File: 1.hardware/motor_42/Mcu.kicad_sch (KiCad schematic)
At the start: 0 parts

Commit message: 중간 저장
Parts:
- added U1: STM32F103CBTx, Package_QFP:LQFP-48_7x7mm_P0.5mm, symbol MCU_ST_STM32F1:STM32F103CBTx
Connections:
- new net: U1.23 (VSS), U1.35 (VSS), U1.47 (VSS)
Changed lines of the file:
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@@
 (kicad_sch
-	(version 20231120)
+	(version 20250114)
 	(generator "eeschema")
-	(generator_version "8.0")
+	(generator_version "9.0")
 	(paper "A4")
+	(symbol
+		(lib_id "MCU_ST_STM32F1:STM32F103CBTx")
+		(at 154.94 92.71 0)
+		(unit 1)
+		(exclude_from_sim no)
+		(in_bom yes)
+		(on_board yes)
+		(dnp no)
+		(fields_autoplaced yes)
+		(property "Reference" "U1"
+			(at 159.6233 133.35 0)
+			(effects
+				(font
+					(size 1.27 1.27)
+				)
+				(justify left)
+			)
+		)
+		(property "Value" "STM32F103CBTx"
+			(at 159.6233 135.89 0)
+			(effects
+				(font
+					(size 1.27 1.27)
+				)
+				(justify left)
+			)
+		)
+		(property "Footprint" "Package_QFP:LQFP-48_7x7mm_P0.5mm"
+			(at 139.7 130.81 0)
+			(effects
+				(font
+					(size 1.27 1.27)
+				)
+				(justify right)
+				(hide yes)
+			)
+		)
+		(property "Datasheet" "https://www.st.com/resource/en/datasheet/stm32f103cb.pdf"
+			(at 154.94 92.71 0)
+			(effects
+				(font
+					(size 1.27 1.27)
+				)
+				(hide yes)
+			)
+		)
+		(property "Description" "STMicroelectronics Arm Cortex-M3 MCU, 128KB flash, 20KB RAM, 72 MHz, 2.0-3.6V, 37 GPIO, LQFP48"
+			(at 154.94 92.71 0)
+			(effects
+				(font
+					(size 1.27 1.27)
+				)
+				(hide yes)
+			)
+		)
+		(pin "18"
+		)
+		(pin "43"
+		)
+		(pin "39"
+		)
+		(pin "24"
+		)
+		(pin "36"
+		)
+		(pin "47"
+		)
+		(pin "1"
+		)
+		(pin "46"
+		)
+		(pin "45"
+		)
+		(pin "27"
+		)
+		(pin "8"
+		)
+		(pin "28"
+		)
+		(pin "21"
+		)
+		(pin "26"
+		)
+		(pin "6"
+		)
+		(pin "3"
+		)
+		(pin "4"
+		)
+		(pin "2"
+		)
+		(pin "19"
+		)
+		(pin "40"
+		)
+		(pin "41"
+		)
+		(pin "5"
+		)
+		(pin "42"
+		)
+		(pin "44"
+		)
+		(pin "7"
+		)
+		(pin "20"
+		)
+		(pin "22"
+		)
+		(pin "25"
+		)
+		(pin "23"
+		)
+		(pin "35"
+		)
+		(pin "48"
+		)
+		(pin "13"
+		)
+		(pin "32"
+		)
+		(pin "31"
+		)
+		(pin "29"
+		)
+		(pin "14"
+		)
+		(pin "17"
+		)
+		(pin "34"
+		)
+		(pin "16"
+		)
+		(pin "38"
+		)
+		(pin "15"
+		)
+		(pin "11"
+		)
+		(pin "30"
+		)
+		(pin "10"
+		)
+		(pin "12"
+		)
+		(pin "33"
+		)
+		(pin "37"
+		)
+		(pin "9"
+		)
+		(instances
+			(project ""
+				(path "/3c5de6a8-6840-43a5-a2fb-24dbb7f0450d/91ecfca5-1fde-4bfb-b396-1bb710e5b1bd"
+					(reference "U1")
+					(unit 1)
+				)
+			)
+		)
+	)
 )

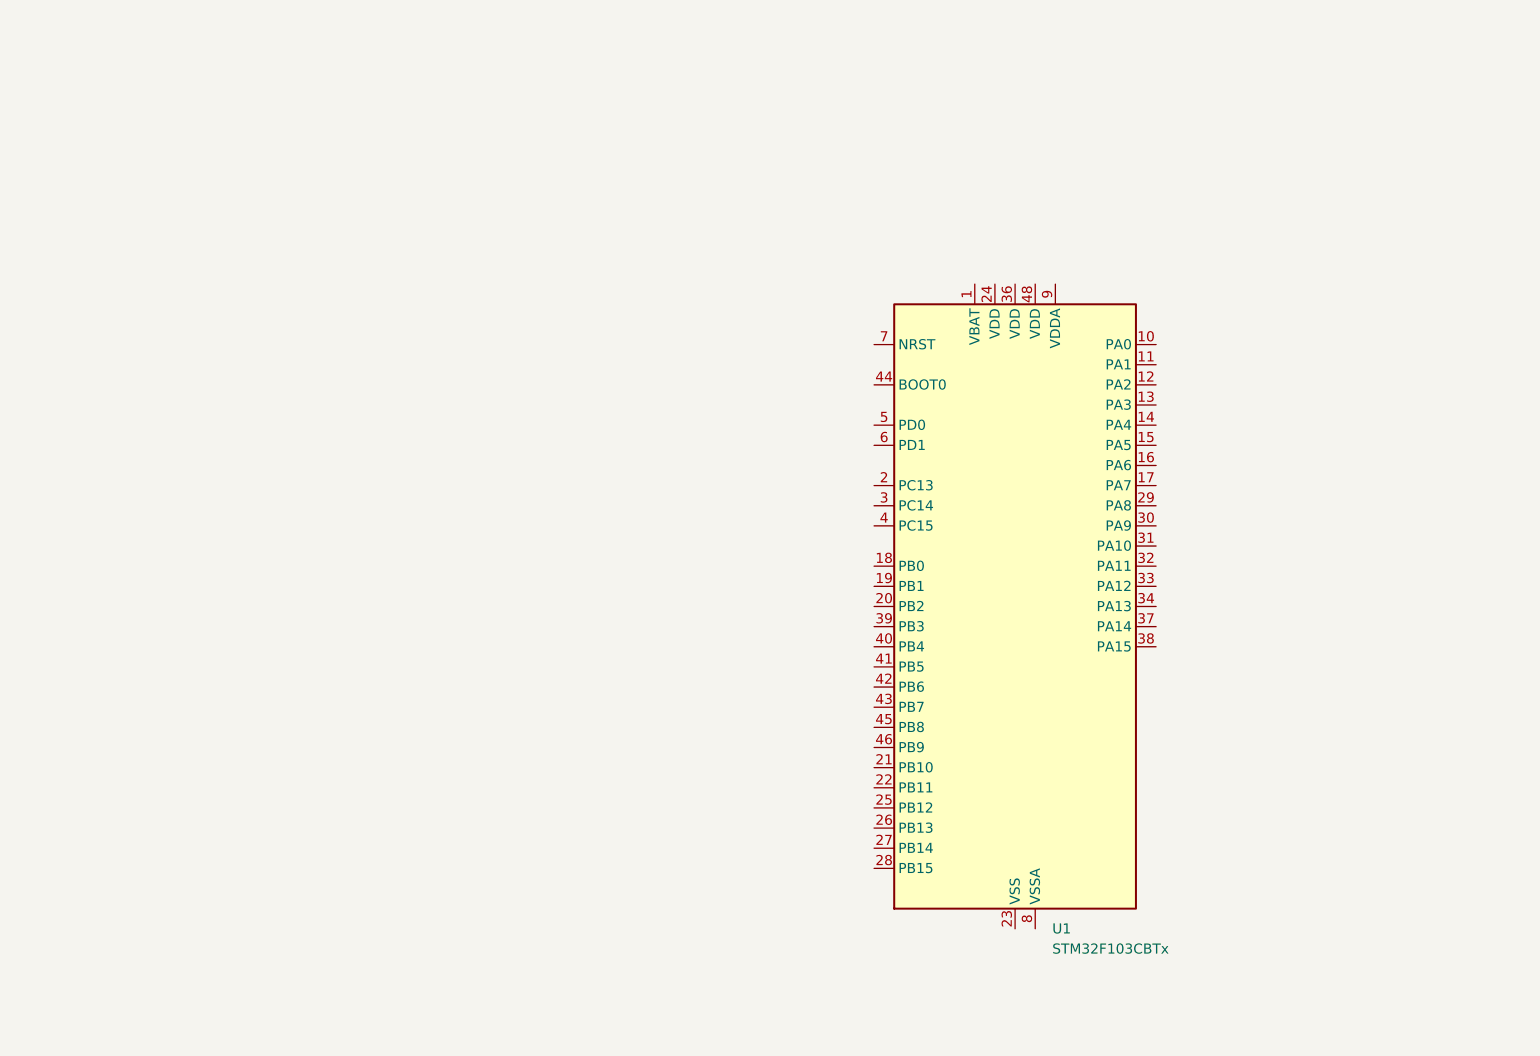
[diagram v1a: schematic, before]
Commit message: 중간 저장
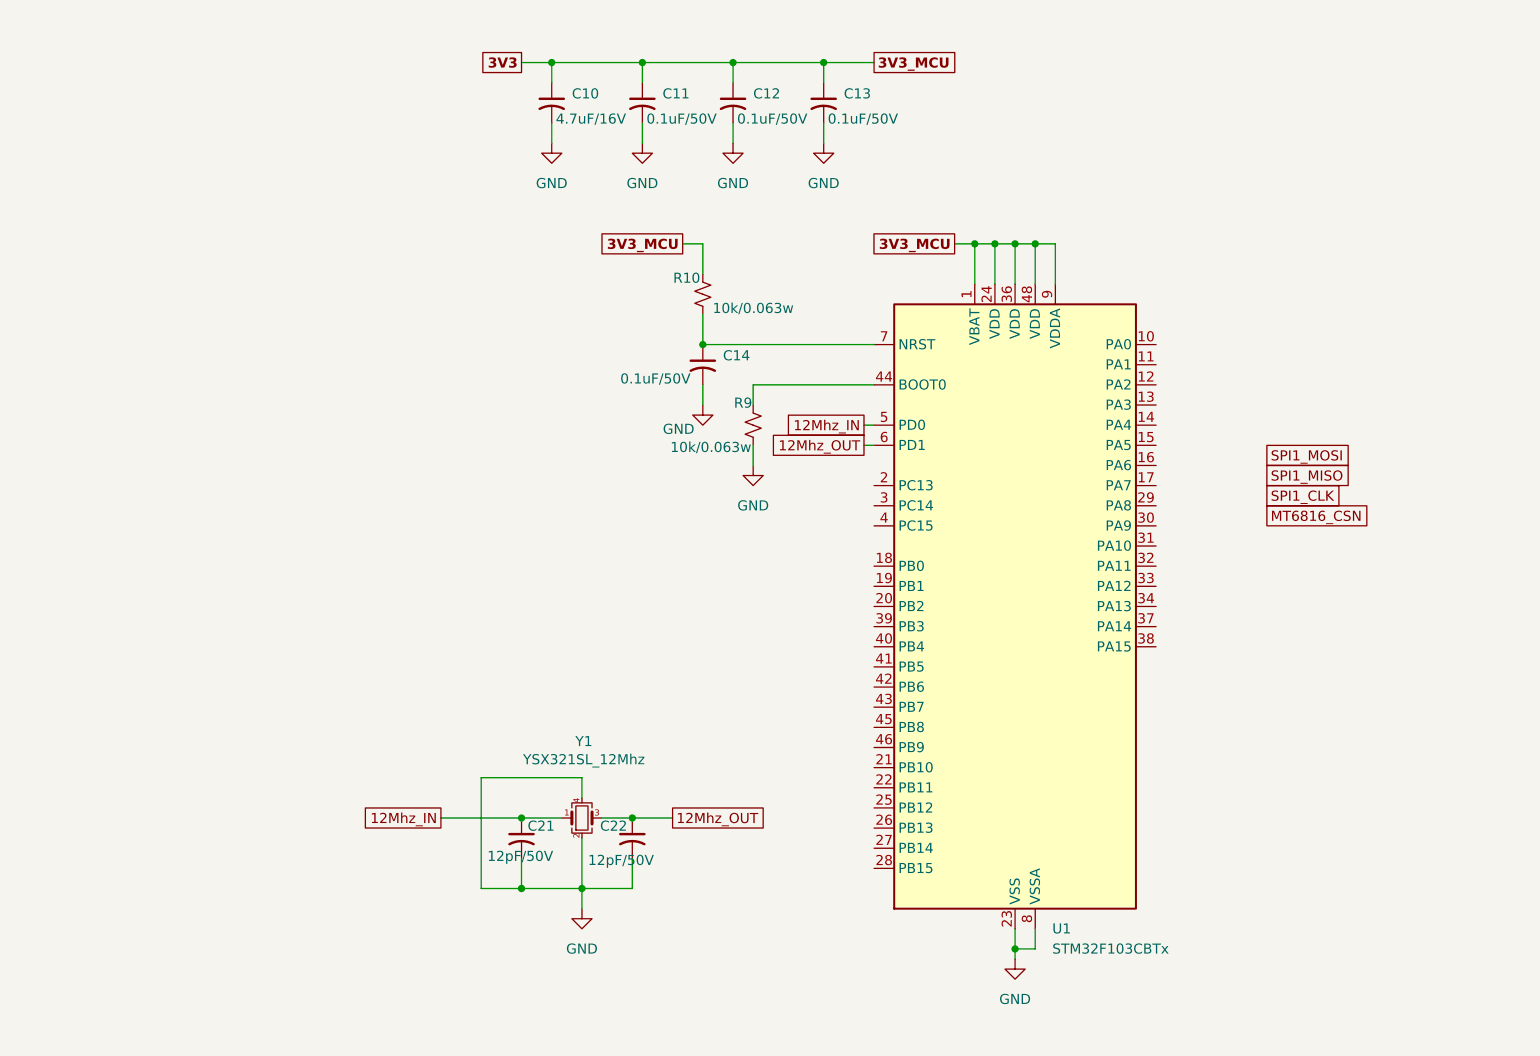
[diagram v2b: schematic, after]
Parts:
- added C10: 4.7uF/16V, symbol Device:C_Small_US
- added C11, C12, C13, C14: 0.1uF/50V, symbol Device:C_Small_US
- added C21, C22: 12pF/50V, symbol Device:C_Small_US
- added R10, R9: 10k/0.063w, symbol Device:R_Small_US
- added Y1: YSX321SL_12Mhz, symbol Device:Crystal_GND24_Small
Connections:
- net 3V3: now reaches U1.1 (VBAT)
- net 3V3: now also U1.24 (VDD), U1.36 (VDD), U1.48 (VDD), U1.9 (VDDA), C10.1, C11.1, C12.1, C13.1, R10.2
- net GND: now reaches U1.23 (VSS), U1.35 (VSS), U1.47 (VSS)
- net GND: now also U1.8 (VSSA), C10.2, C11.2, C12.2, C13.2, C14.2, C21.2, C22.2, R9.2, Y1.2, Y1.4
- net at U1.44 (BOOT0): now also R9.1
- net 12Mhz_IN: now reaches U1.5 (PD0)
- net 12Mhz_IN: now also C21.1, Y1.1
- net 12Mhz_OUT: now reaches U1.6 (PD1)
- net 12Mhz_OUT: now also C22.1, Y1.3
- net at U1.7 (NRST): now also C14.1, R10.1

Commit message: 중간 저장
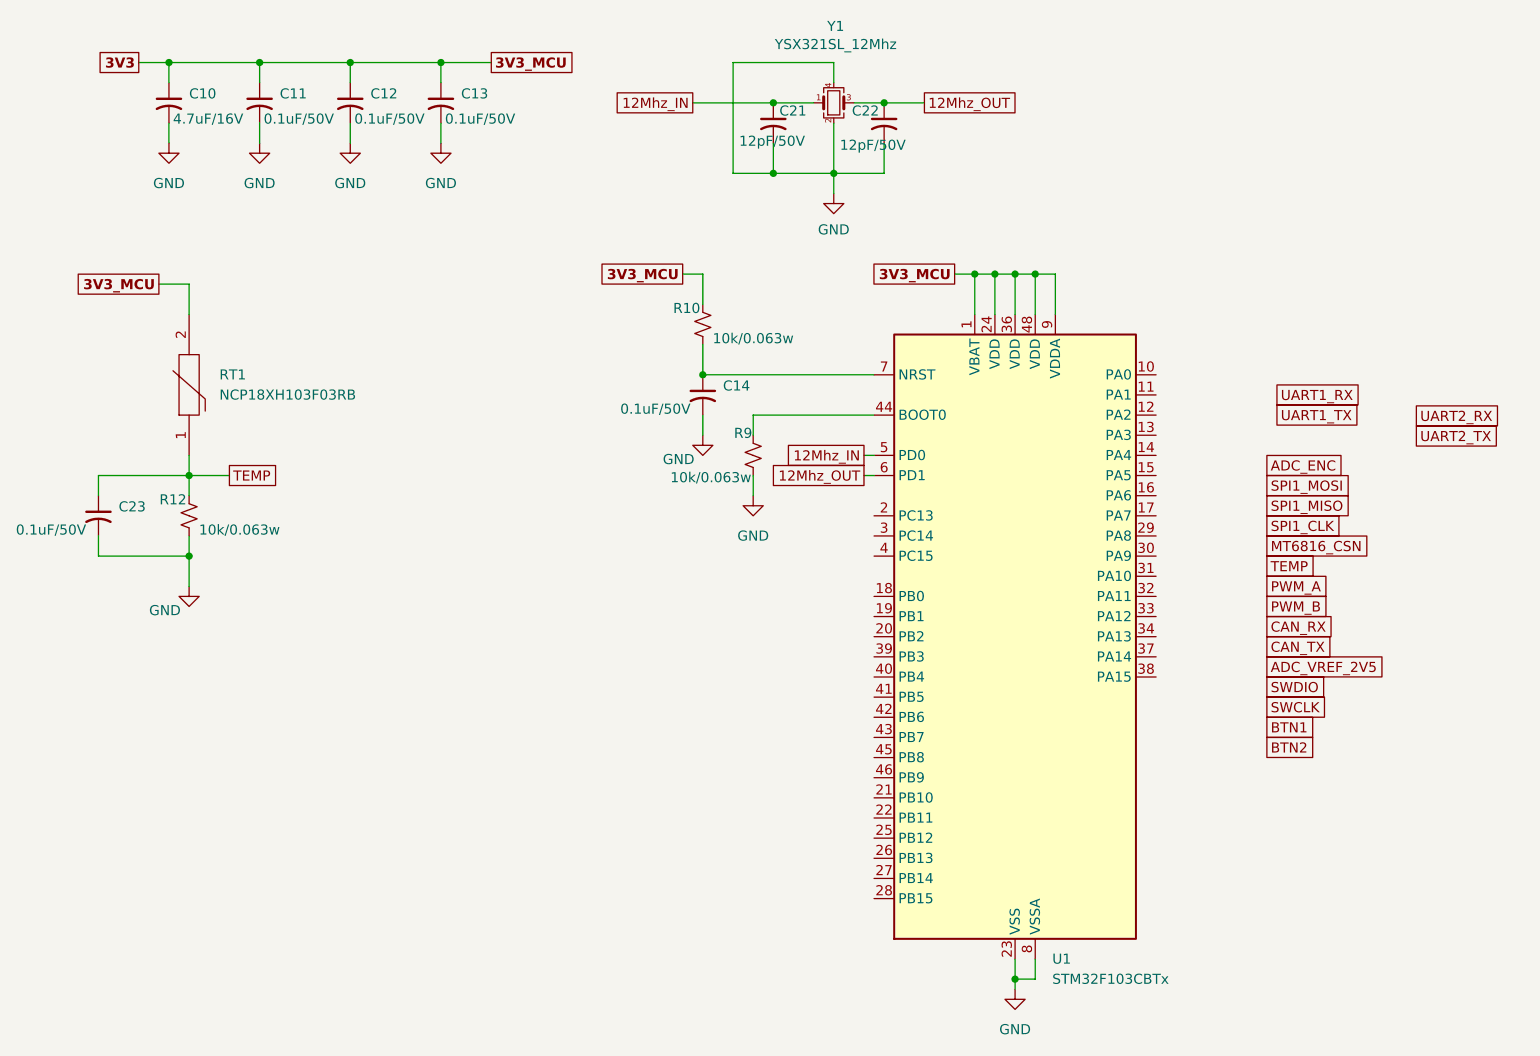
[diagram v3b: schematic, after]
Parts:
- added C23: 0.1uF/50V, symbol Device:C_Small_US
- added R12: 10k/0.063w, symbol Device:R_Small_US
- added RT1: NCP18XH103F03RB, THRMC1608X95N, symbol SamacSys_Parts:NCP18XH103F03RB
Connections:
- net 3V3: now also RT1.2
- net GND: now also C23.2, R12.1
- new net TEMP: C23.1, R12.2, RT1.1
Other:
- moved on the sheet: C10, C11, C12, C13, C14, C21, C22, R10, R9, U1, Y1
